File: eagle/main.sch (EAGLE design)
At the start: 43 parts, among them Q1 SQJ886EP, U1 LTC3789EGNPBF

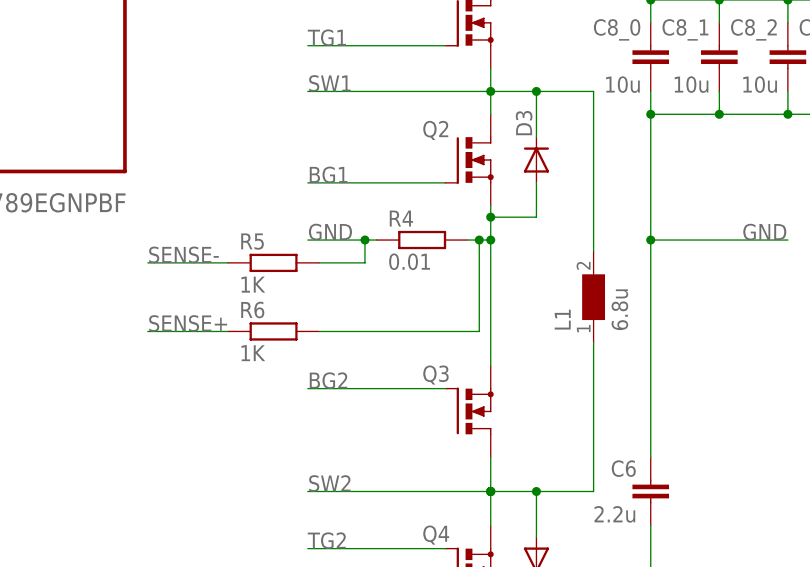
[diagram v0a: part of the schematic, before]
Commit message: [ update ] sch
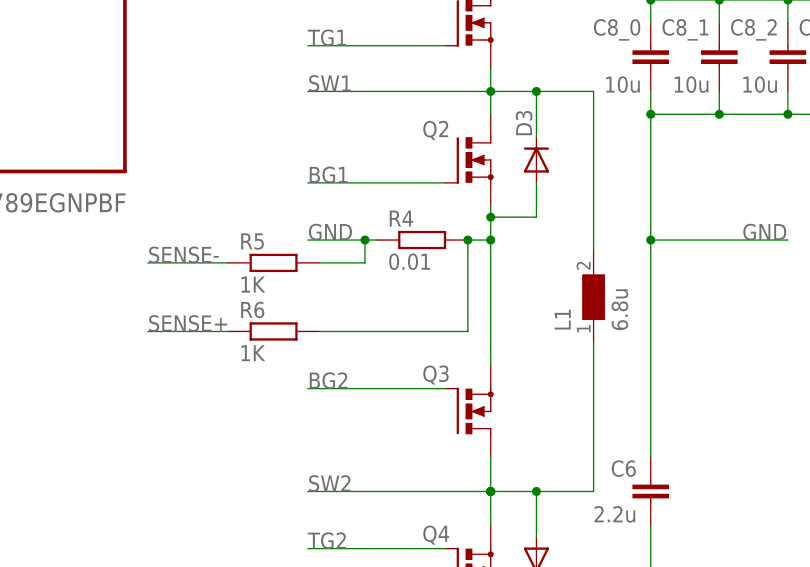
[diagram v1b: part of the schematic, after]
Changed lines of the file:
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@@
 <part name="C6" library="rcl" deviceset="C-EU" device="C1206K" value="2.2u"/>
 <part name="C8_0" library="rcl" deviceset="C-EU" device="C1206K" value="10u"/>
-<part name="R4" library="resistor" deviceset="R-EU_" device="R1206" value="0.01"/>
 <part name="C12" library="rcl" deviceset="C-EU" device="C1206K" value="0.22u"/>
 <part name="C13" library="rcl" deviceset="C-EU" device="C1206K" value="0.22u"/>
@@
 <part name="CON_PIN" library="con-ptr500" deviceset="AK300/2" device=""/>
 <part name="CON_POUT" library="con-ptr500" deviceset="AK300/2" device=""/>
+<part name="R4" library="resistor" deviceset="R-EU_" device="R1206" value="0.01"/>
 </parts>
 <sheets>
@@
 <attribute name="VALUE" x="156.464" y="42.291" size="1.778" layer="96" align="top-right"/>
 </instance>
-<instance part="R4" gate="G$1" x="132.08" y="24.13"/>
 <instance part="C12" gate="G$1" x="173.99" y="114.3" smashed="yes" rot="R90">
 <attribute name="NAME" x="169.799" y="115.824" size="1.778" layer="95" rot="R180" align="top-right"/>
@@
 <instance part="CON_POUT" gate="-1" x="10.16" y="5.08"/>
 <instance part="CON_POUT" gate="-2" x="10.16" y="0"/>
+<instance part="R4" gate="G$1" x="132.08" y="24.13"/>
 </instances>
 <busses>
@@
 </segment>
 <segment>
-<pinref part="R4" gate="G$1" pin="1"/>
 <wire x1="127" y1="24.13" x2="125.73" y2="24.13" width="0.1524" layer="91"/>
 <label x="119.38" y="24.13" size="1.778" layer="95"/>
@@
 <wire x1="125.73" y1="21.59" x2="120.65" y2="21.59" width="0.1524" layer="91"/>
 <pinref part="R5" gate="G$1" pin="2"/>
+<pinref part="R4" gate="G$1" pin="1"/>
 </segment>
 <segment>
@@
 <segment>
 <wire x1="139.7" y1="10.16" x2="139.7" y2="24.13" width="0.1524" layer="91"/>
-<pinref part="R4" gate="G$1" pin="2"/>
 <wire x1="139.7" y1="24.13" x2="139.7" y2="26.67" width="0.1524" layer="91"/>
 <wire x1="139.7" y1="26.67" x2="139.7" y2="27.94" width="0.1524" layer="91"/>
-<wire x1="137.16" y1="24.13" x2="138.43" y2="24.13" width="0.1524" layer="91"/>
 <junction x="139.7" y="24.13"/>
-<wire x1="138.43" y1="24.13" x2="139.7" y2="24.13" width="0.1524" layer="91"/>
-<wire x1="138.43" y1="24.13" x2="138.43" y2="13.97" width="0.1524" layer="91"/>
-<junction x="138.43" y="24.13"/>
-<wire x1="138.43" y1="13.97" x2="120.65" y2="13.97" width="0.1524" layer="91"/>
+<wire x1="137.16" y1="24.13" x2="139.7" y2="24.13" width="0.1524" layer="91"/>
+<wire x1="137.16" y1="24.13" x2="137.16" y2="13.97" width="0.1524" layer="91"/>
+<wire x1="137.16" y1="13.97" x2="120.65" y2="13.97" width="0.1524" layer="91"/>
 <wire x1="139.7" y1="26.67" x2="144.78" y2="26.67" width="0.1524" layer="91"/>
 <junction x="139.7" y="26.67"/>
@@
 <pinref part="Q2" gate="G$1" pin="S"/>
 <pinref part="Q3" gate="G$1" pin="S"/>
-</segment>
-</net>
+<pinref part="R4" gate="G$1" pin="2"/>
+<junction x="137.16" y="24.13"/>
+</segment>
+</net>
